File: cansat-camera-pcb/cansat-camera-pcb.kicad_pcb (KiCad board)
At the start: 8 copper layers, 50 x 50 mm, 60 parts, among them IC1 W9825G6JB-6I, IC2 TLV74315PDBVR, J3 Conn_01x05_Socket, J4 Conn_02x10_Odd_Even, J5 Conn_02x10_Odd_Even, J6 OV5640, SW2 SW_Push, U2 AP2112K-3.3, U4 STM32H743ZITx, U6 TLV74328PDBVR, Y1 24MHz

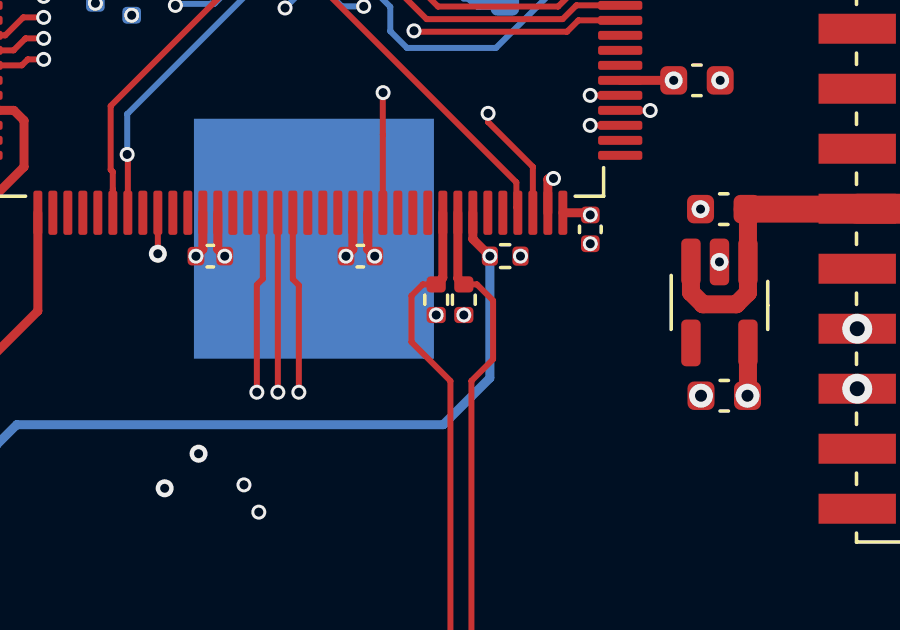
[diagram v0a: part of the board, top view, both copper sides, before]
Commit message: -
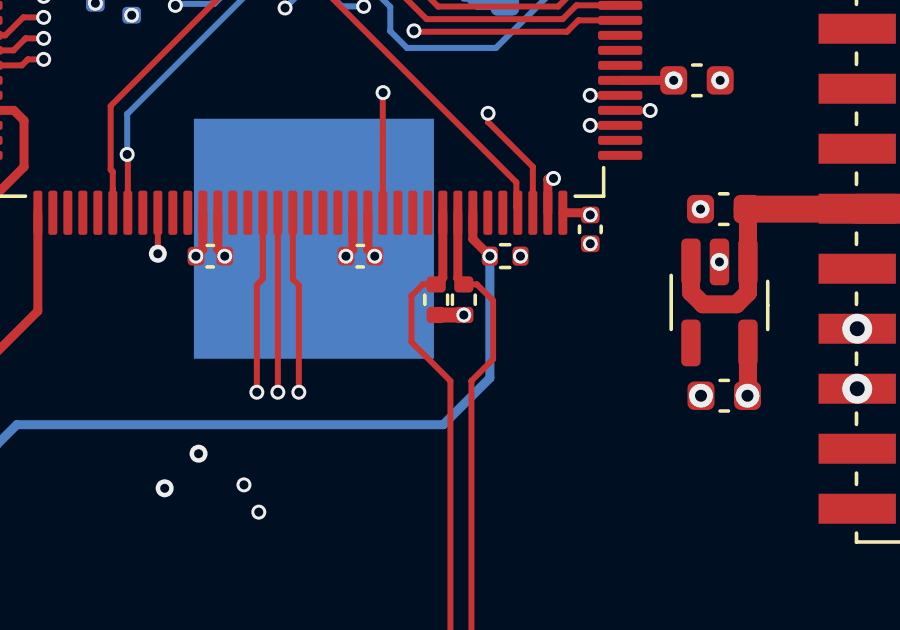
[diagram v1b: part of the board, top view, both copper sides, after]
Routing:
- net +3.3V: track 58.4 -> 59.3 mm, vias 38 -> 37
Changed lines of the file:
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@@
+	)
+	(segment
+		(start 78 130.162)
+		(end 78.921 130.162)
+		(width 0.5)
+		(layer "F.Cu")
+		(net 6)
 	)
 	(segment
@@
 		(net 6)
 	)
-	(via blind
-		(at 78 130.162)
-		(size 0.5)
-		(drill 0.3)
-		(layers "F.Cu" "In4.Cu")
-		(free yes)
-		(net 6)
-	)
 	(via
 		(at 59.99 137.0265)
@@
 		(net 6)
 	)
-	(via blind
+	(via
 		(at 78.921 130.162)
 		(size 0.5)
 		(drill 0.3)
-		(layers "F.Cu" "In4.Cu")
-		(free yes)
-		(net 6)
+		(layers "F.Cu" "B.Cu")
+		(free yes)
+		(net 6)

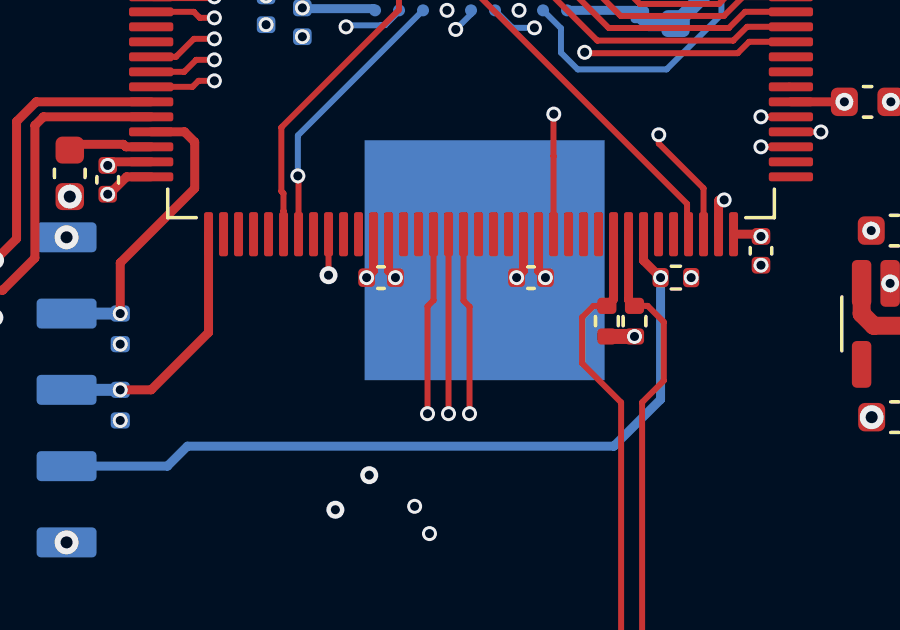
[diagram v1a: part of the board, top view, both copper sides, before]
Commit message: Update cansat-camera-pcb.kicad_pcb
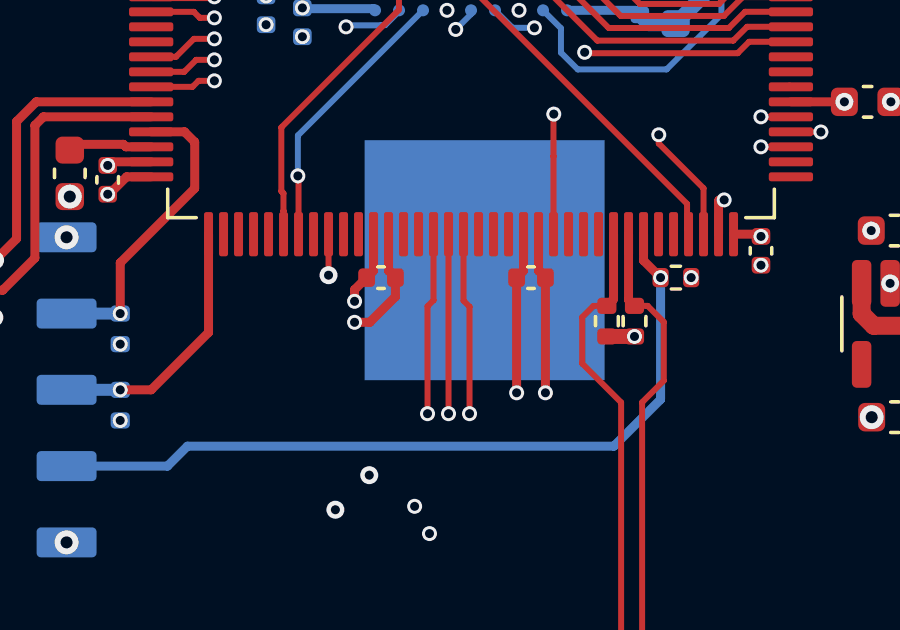
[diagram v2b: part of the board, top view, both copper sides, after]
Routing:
- net +3.3V: track 59.3 -> 65.5 mm
- net GND: track 33.6 -> 38.4 mm
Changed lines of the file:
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@@
-	)
-	(segment
-		(start 70.222012 126.7535)
-		(end 70.222012 127.971)
-		(width 0.3)
-		(layer "F.Cu")
-		(net 1)
 	)
 	(segment
@@
 	)
 	(segment
+		(start 69.59 128.603012)
+		(end 70.222012 127.971)
+		(width 0.3)
+		(layer "F.Cu")
+		(net 1)
+	)
+	(segment
 		(start 81.722012 125.642012)
 		(end 81.754024 125.61)
@@
 	)
 	(segment
-		(start 70.222012 127.971)
-		(end 69.992012 128.201)
-		(width 0.3)
-		(layer "F.Cu")
-		(net 1)
-	)
-	(segment
 		(start 85.352012 117.341)
 		(end 85.582012 117.571)
@@
 		(start 84.134512 109.841)
 		(end 86.352012 109.841)
+		(width 0.3)
+		(layer "F.Cu")
+		(net 1)
+	)
+	(segment
+		(start 69.59 128.99)
+		(end 69.59 128.603012)
 		(width 0.3)
 		(layer "F.Cu")
@@
 	)
 	(segment
+		(start 70.222012 127.971)
+		(end 70.222012 126.7535)
+		(width 0.3)
+		(layer "F.Cu")
+		(net 1)
+	)
+	(segment
 		(start 75.222012 104.211)
 		(end 75.452012 103.981)
@@
 		(start 86.352012 109.841)
 		(end 86.582012 109.611)
+		(width 0.3)
+		(layer "F.Cu")
+		(net 1)
+	)
+	(segment
+		(start 74.992012 128.201)
+		(end 74.992012 132.04)
 		(width 0.3)
 		(layer "F.Cu")
@@
 	)
 	(via blind
-		(at 69.992012 128.201)
+		(at 69.59 128.99)
 		(size 0.5)
 		(drill 0.3)
@@
 	)
 	(via blind
-		(at 74.992012 128.201)
+		(at 74.992012 132.04)
 		(size 0.5)
 		(drill 0.3)
@@
 	)
 	(segment
-		(start 70.722012 127.971)
-		(end 70.952012 128.201)
-		(width 0.3)
-		(layer "F.Cu")
-		(net 6)
-	)
-	(segment
 		(start 81.222012 104.211)
 		(end 80.992012 103.981)
@@
 	)
 	(segment
+		(start 69.63 129.69)
+		(end 70.1 129.69)
+		(width 0.3)
+		(layer "F.Cu")
+		(net 6)
+	)
+	(segment
 		(start 62.809512 124.841)
 		(end 61.990272 124.841)
@@
 	)
 	(segment
-		(start 70.722012 126.7535)
+		(start 75.952012 128.201)
+		(end 75.952012 132.04)
+		(width 0.3)
+		(layer "F.Cu")
+		(net 6)
+	)
+	(segment
+		(start 70.952012 128.201)
 		(end 70.722012 127.971)
 		(width 0.3)
@@
 		(start 84.134512 110.341)
 		(end 86.352012 110.341)
+		(width 0.3)
+		(layer "F.Cu")
+		(net 6)
+	)
+	(segment
+		(start 70.952012 128.837988)
+		(end 70.952012 128.201)
 		(width 0.3)
 		(layer "F.Cu")
@@
 	)
 	(segment
+		(start 70.1 129.69)
+		(end 70.952012 128.837988)
+		(width 0.3)
+		(layer "F.Cu")
+		(net 6)
+	)
+	(segment
 		(start 74.722012 104.211)
 		(end 74.492012 103.981)
@@
 	)
 	(segment
+		(start 70.722012 127.971)
+		(end 70.722012 126.7535)
+		(width 0.3)
+		(layer "F.Cu")
+		(net 6)
+	)
+	(segment
 		(start 82.222012 126.7535)
 		(end 83.0635 126.7535)
@@
 	)
 	(via blind
-		(at 70.952012 128.201)
+		(at 69.59 129.69)
 		(size 0.5)
 		(drill 0.3)
@@
 	)
 	(via blind
-		(at 75.952012 128.201)
-		(size 0.5)
-		(drill 0.3)
+		(at 75.952012 132.04)
+		(size 0.5)
+		(drill 0.3)
